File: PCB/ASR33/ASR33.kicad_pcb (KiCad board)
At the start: 2 copper layers, 70 x 70 mm, 41 parts, among them J2 DC, J3 Power, J4 RUN, J5 Tx, J6 Rx, J7 USB-C-Socket-V, J8 TC2030-USB-NL-DS, Q1 NX7002AK, SW1 SW_Push, U1 MD8942, U3 NCR402U, U4 NCR402U, U5 LTV-356T, U7 QR, U8 ESP32-S3-MINI-1

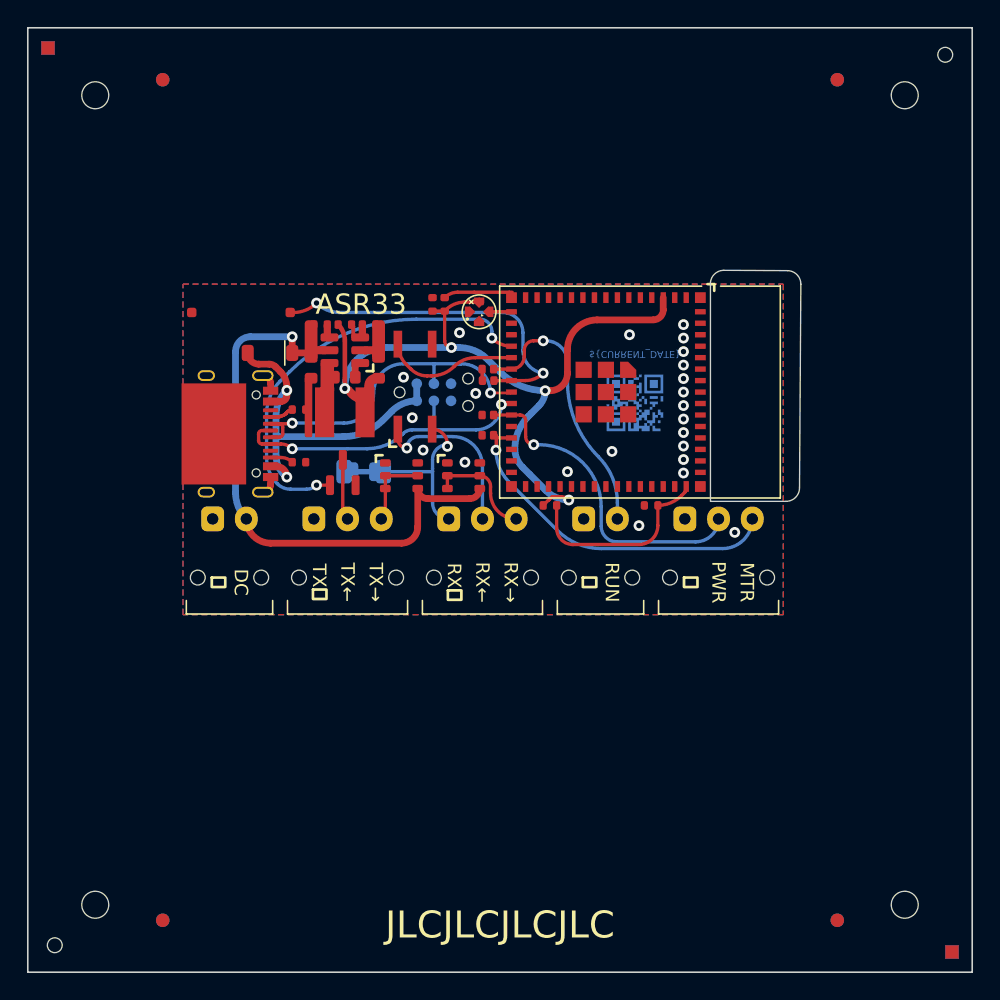
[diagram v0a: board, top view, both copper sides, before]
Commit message: New images
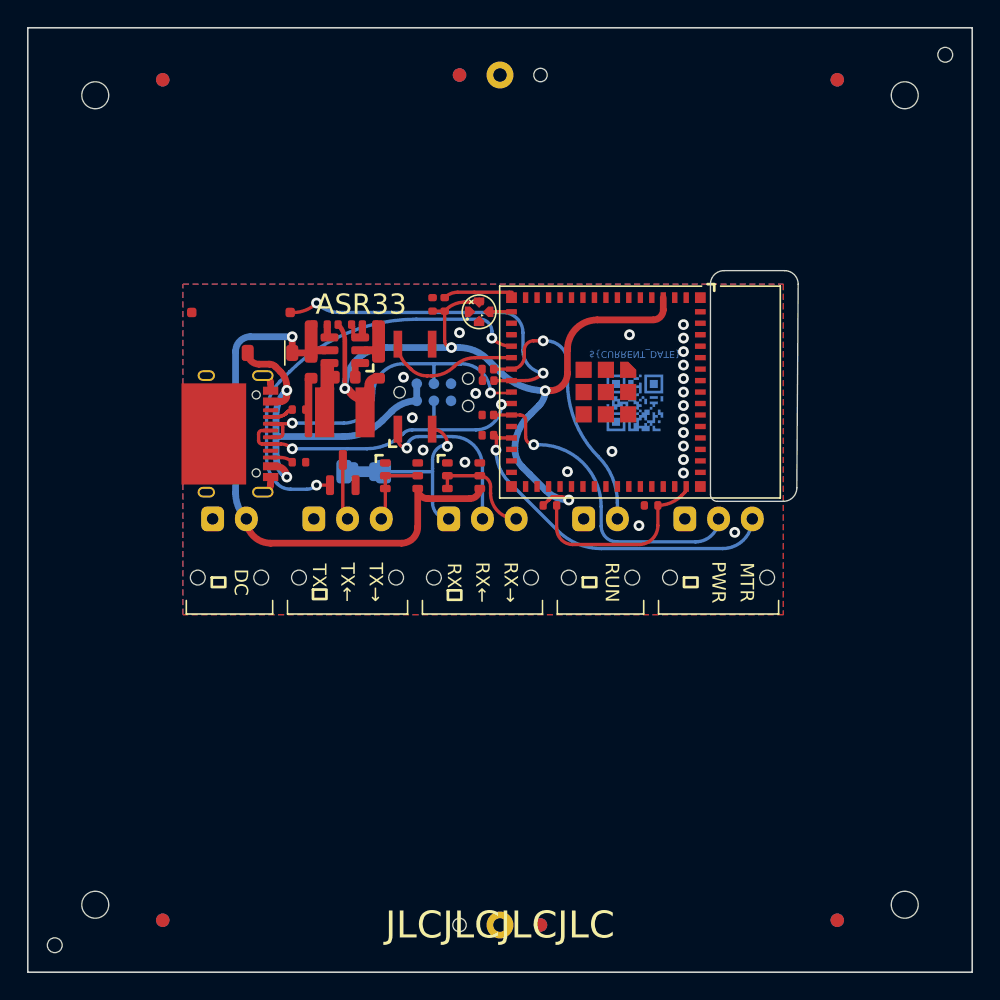
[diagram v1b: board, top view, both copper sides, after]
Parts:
- removed REF**: Shadow, RevK:Shadow

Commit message: PCB Update
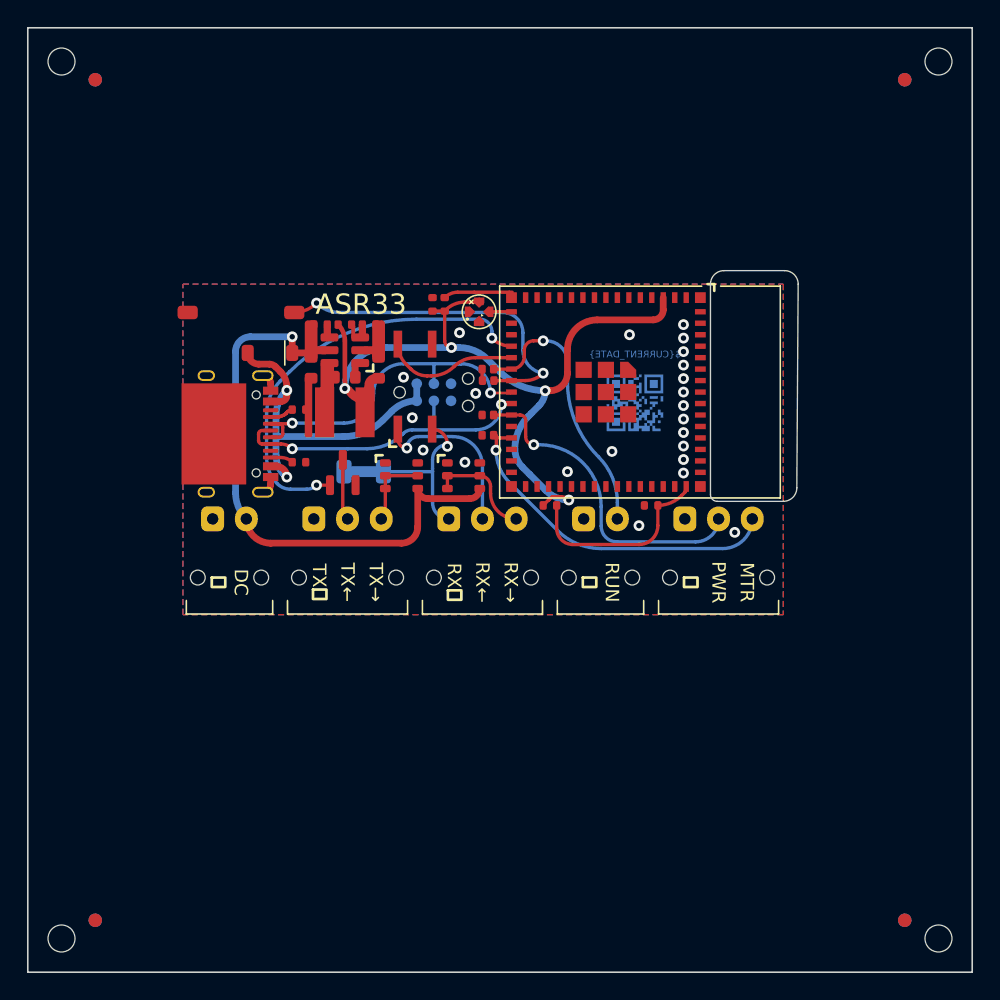
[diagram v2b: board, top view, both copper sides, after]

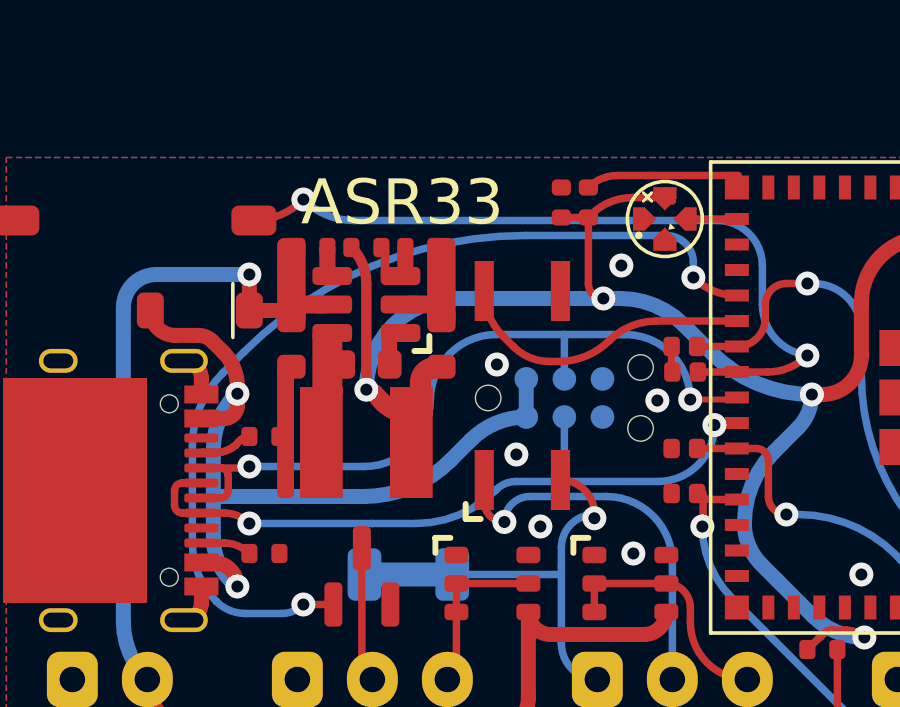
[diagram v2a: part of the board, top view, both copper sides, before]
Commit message: Image and new tc2030
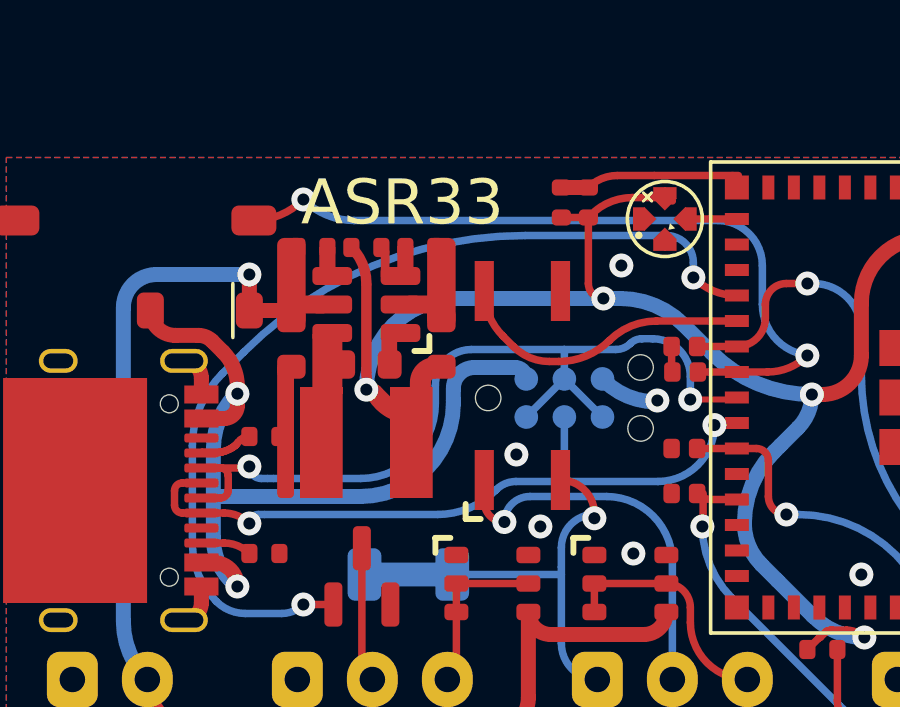
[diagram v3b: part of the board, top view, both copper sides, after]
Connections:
- J8 pad 2: VBUS -> D-
- J8 pad 6: GND -> D-
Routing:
- net D-: track 25.7 -> 29.3 mm
- net GND: track 9.31 -> 12.3 mm, vias 23 -> 22
- net VBUS: track 27.3 -> 28.0 mm
